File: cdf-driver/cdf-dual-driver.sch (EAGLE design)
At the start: 30 parts, among them IC1 R-789.0-0.5, IC2 UCC27423, Q1 FDD8424H, Q2 FDD8424H

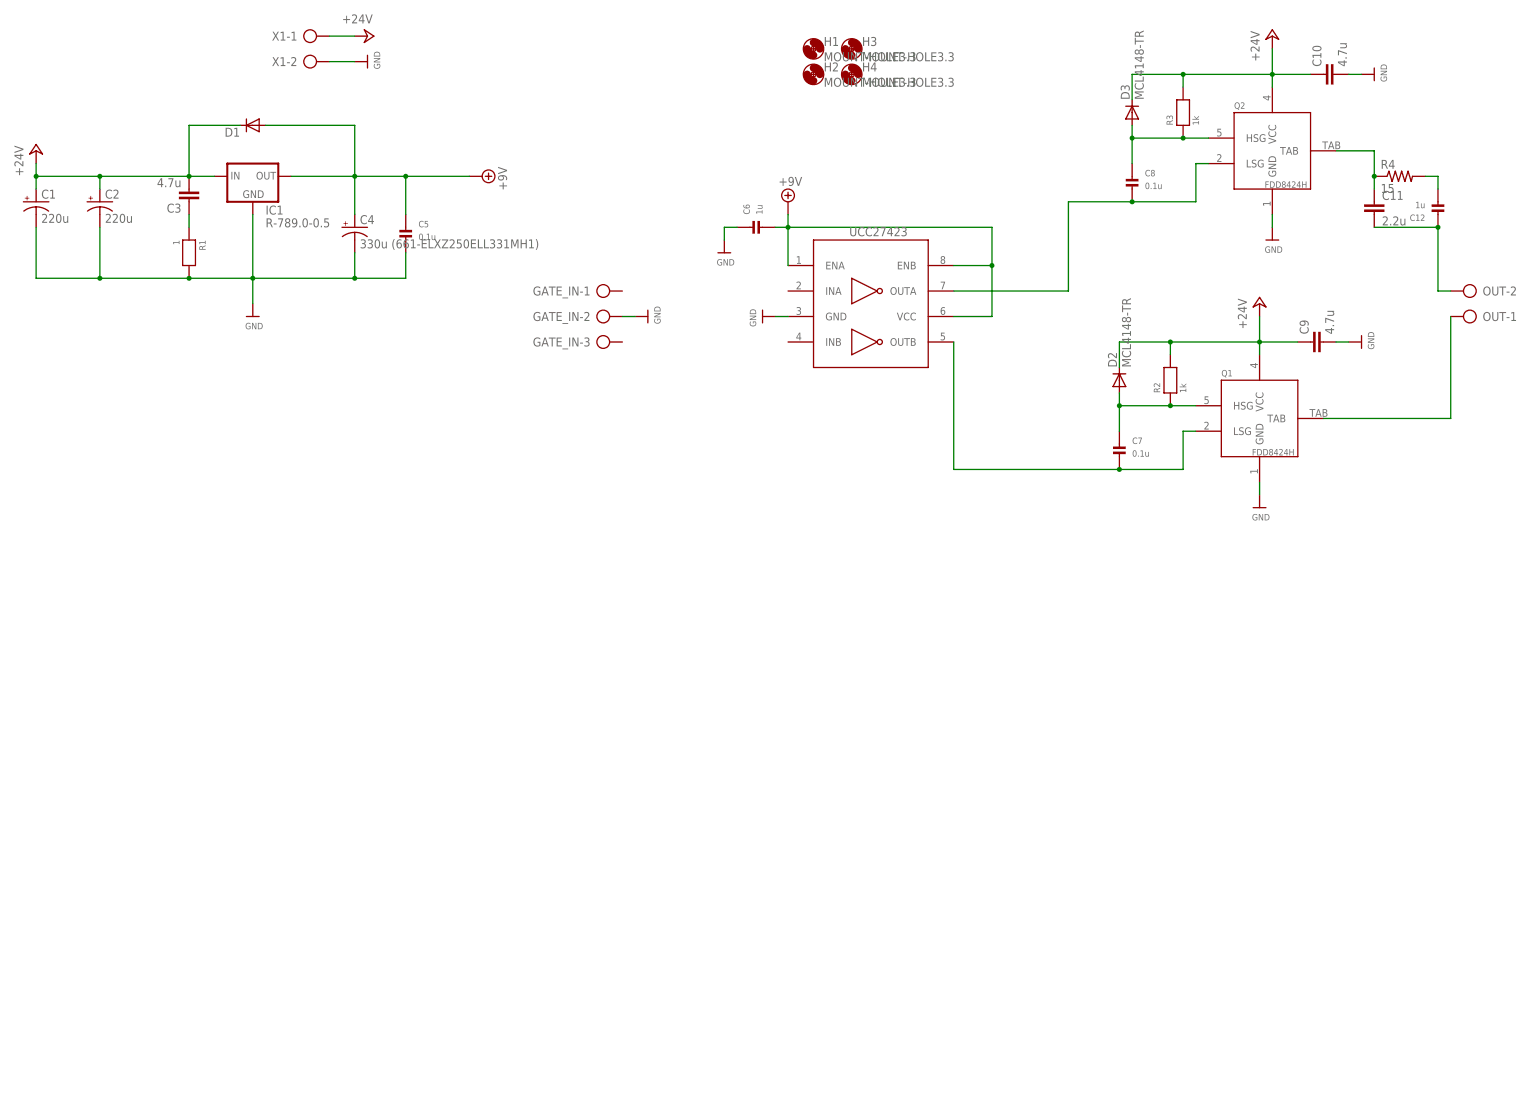
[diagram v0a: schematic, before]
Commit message: wip
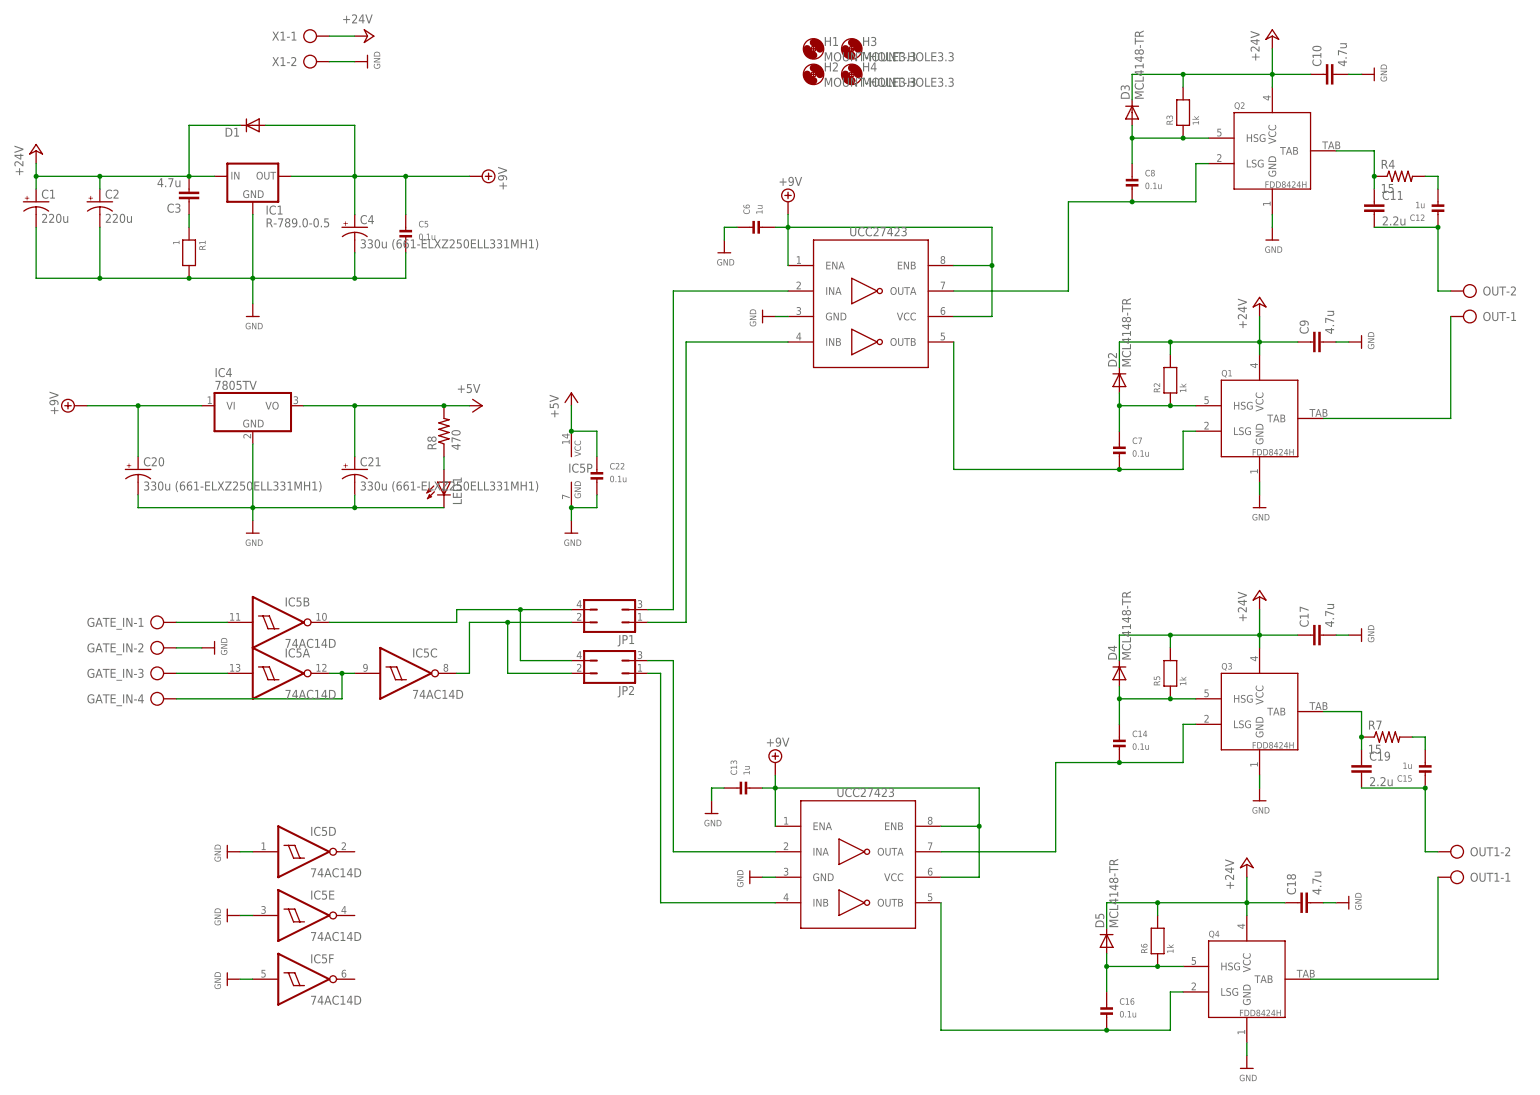
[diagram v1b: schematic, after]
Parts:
- added C13, C15: 1u, microbuilder:CAP_CERAMIC1206
- added C14, C16, C22: 0.1u, microbuilder:CAP_CERAMIC0805
- added C17, C18: 4.7u, rcl:C-EUC1210
- added C19: 2.2u, rcl:C-EUC1210
- added C20, C21: 330u (661-ELXZ250ELL331MH1), rcl:CPOL-USE3.5-8
- added D4, D5: MCL4148-TR, diode:DIODE-MICROMELF-W
- added IC3: UCC27423, keves:UCC27423
- added IC4: 7805TV, linear:7805TV
- added IC5: 74AC14D, 74xx-eu:74AC14D
- added JP1, JP2: (no value), jumper:JP2Q
- added LED1: (no value), led:LED5MM
- added OUT1: (no value), con-ptr500:AK500/2
- added Q3, Q4: FDD8424H, keves:FDD8424H
- added R5, R6: 1k, microbuilder:RESISTOR0805
- added R7: 15, rcl:R-US_R1210
- added R8: 470, rcl:R-US_0204/7
- GATE_IN: device con-ptr500:AK500/3 -> con-ptr500:AK500/4
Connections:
- new net +5V: C21.+, C22.P$1, IC4.VO, IC5P.VCC, R8.2
- new net N$1: C14.P$2, IC3.OUTA, Q3.LSG
- new net N$12: C19.1, Q3.TAB, R7.1
- new net N$13: C15.P$2, R7.2
- new net N$14: C15.P$1, C19.2, OUT1-2.KL
- new net N$15: C16.P$2, IC3.OUTB, Q4.LSG
- new net N$16: C16.P$1, D5.A, Q4.HSG, R6.1
- new net N$17: OUT1-1.KL, Q4.TAB
- new net N$18: LED1.A, R8.1
- new net N$19: IC2.INA, JP1.3
- new net N$2: C14.P$1, D4.A, Q3.HSG, R5.1
- new net N$20: IC2.INB, JP1.1
- new net N$21: IC3.INA, JP2.3
- new net N$22: IC3.INB, JP2.1
- new net N$23: GATE_IN-1.KL, IC5B.I
- new net N$24: IC5B.O, JP1.4, JP2.4
- new net N$25: GATE_IN-3.KL, IC5A.I
- new net N$26: GATE_IN-4.KL, IC5A.O, IC5C.I
- new net N$27: IC5C.O, JP1.2, JP2.2
- net +24V: now also C17.1, C18.1, D4.C, D5.C, Q3.VCC, Q4.VCC, R5.2, R6.2
- net +9V: now also C13.P$2, C20.+, IC3.ENA, IC3.ENB, IC3.VCC, IC4.VI
- net GND: now also C13.P$1, C17.2, C18.2, C20.-, C21.-, C22.P$2, IC3.GND, IC4.GND, IC5D.I, IC5E.I, IC5F.I, IC5P.GND, LED1.C, Q3.GND, Q4.GND
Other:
- moved on the sheet: GATE_IN-1, GATE_IN-2, GATE_IN-3
